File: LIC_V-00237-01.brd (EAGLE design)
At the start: 48.5 x 45 mm, 15 parts, among them J1 S4B-PH-SM4-TB

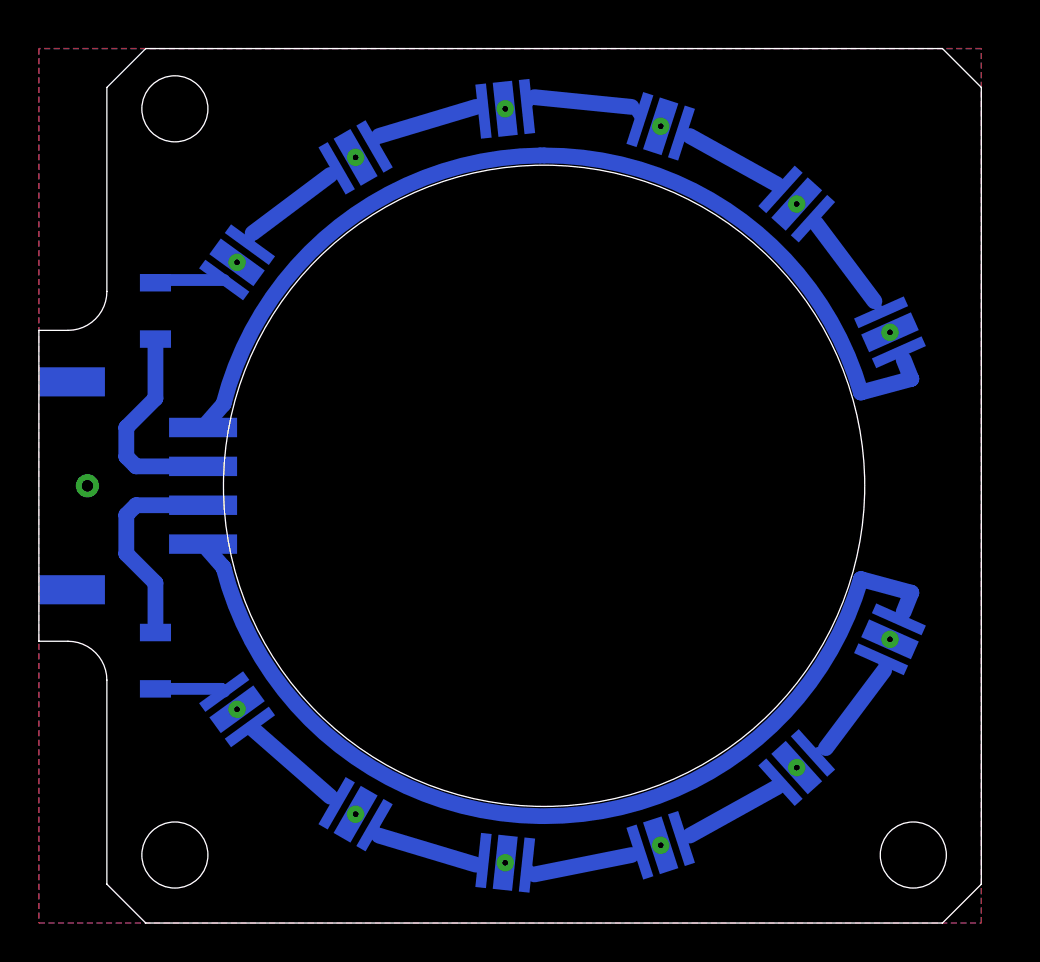
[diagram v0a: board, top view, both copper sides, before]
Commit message: Další verze
Verze pro normální LED
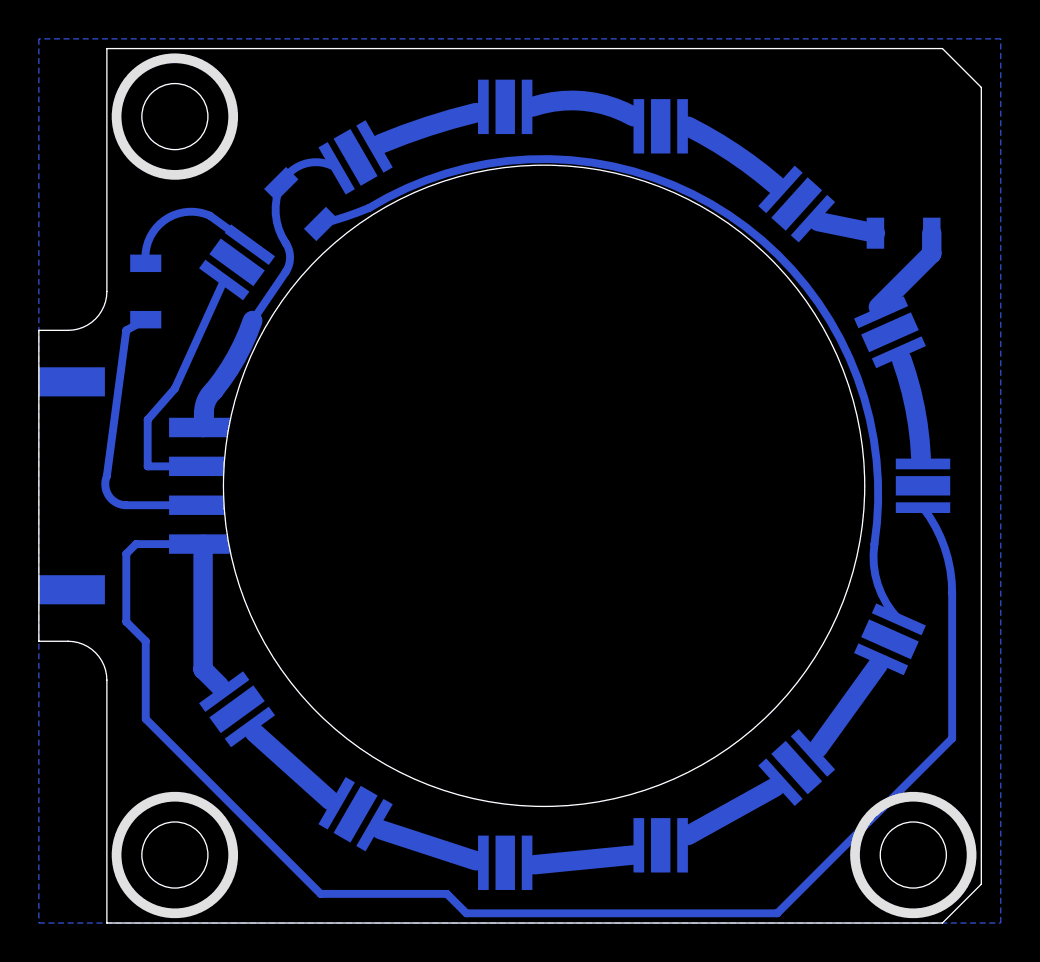
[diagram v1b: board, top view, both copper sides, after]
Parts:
- added D7: OSRAM_LCW_CQ7P.EC-KTLP-5J7K-1-K, led:OSRAM_LCW
- added R3: 2k2, rcl:R1206
- R1, R2: value (none) -> 22R0
- moved R1 38.7 mm to (44.5, 35.5), turned to 0 degrees
- moved D1 33.8 mm to (43.8, 14.6), turned to 294 degrees
- moved D6 33.8 mm to (10.2, 11.0), turned to 54 degrees
- moved R2 24.7 mm to (13.5, 37.0), turned to 45 degrees
- moved D2 22.8 mm to (39.0, 8.00), turned to 318 degrees
- moved D5 22.8 mm to (16.3, 5.60), turned to 30 degrees
- moved D12 8.16 mm to (43.8, 30.4), turned to 246 degrees
- moved D8 8.15 mm to (16.3, 39.4), turned to 150 degrees
- moved D9 8.13 mm to (24.0, 42.0), turned to 180 degrees
- moved D13 8.08 mm to (45.5, 22.5), turned to 270 degrees
- moved D11 8.06 mm to (39.0, 37.0), turned to 222 degrees
- moved D10 8.05 mm to (32.0, 41.0), turned to 180 degrees
- moved D3 8.05 mm to (32.0, 4.00), turned to 0 degrees
- moved D4 8.05 mm to (24.0, 3.10), turned to 0 degrees
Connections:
- new net N$12: D7.A, R3.1
- net 1+: now also D8.A, J1.4; no longer J1.2
- net 1-: now also D13.C
- net 2+: now also J1.2, R3.2; no longer J1.3, R1.2
- net 2-: now also D7.C, J1.3; no longer D13.C, J1.4
- net N$10: now also R1.1; no longer D11.C
- net N$11: now also D11.C, R1.2; no longer D8.A, R1.1
- net THERMAL: now also D7.THERMAL
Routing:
- net 1-: track 46.9 -> 82.6 mm
- net N$6: track 3.60 -> 37.9 mm
- net 2-: track 47.1 -> 13.5 mm
- net N$12: track 0.00 -> 6.65 mm
- net 1+: track 10.8 -> 16.6 mm
- net 2+: track 10.8 -> 14.5 mm
- net N$10: track 5.90 -> 5.25 mm
- removed copper zone on layer 1, net THERMAL
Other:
- outline, holes or cut-outs redrawn
